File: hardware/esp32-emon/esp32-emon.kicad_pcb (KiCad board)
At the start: 2 copper layers, 86 x 35.2 mm, 11 parts, among them J1 SJ-3523-SMT-TR, J2 SJ-3523-SMT-TR, U1 ESP32-DEVKIT-V1

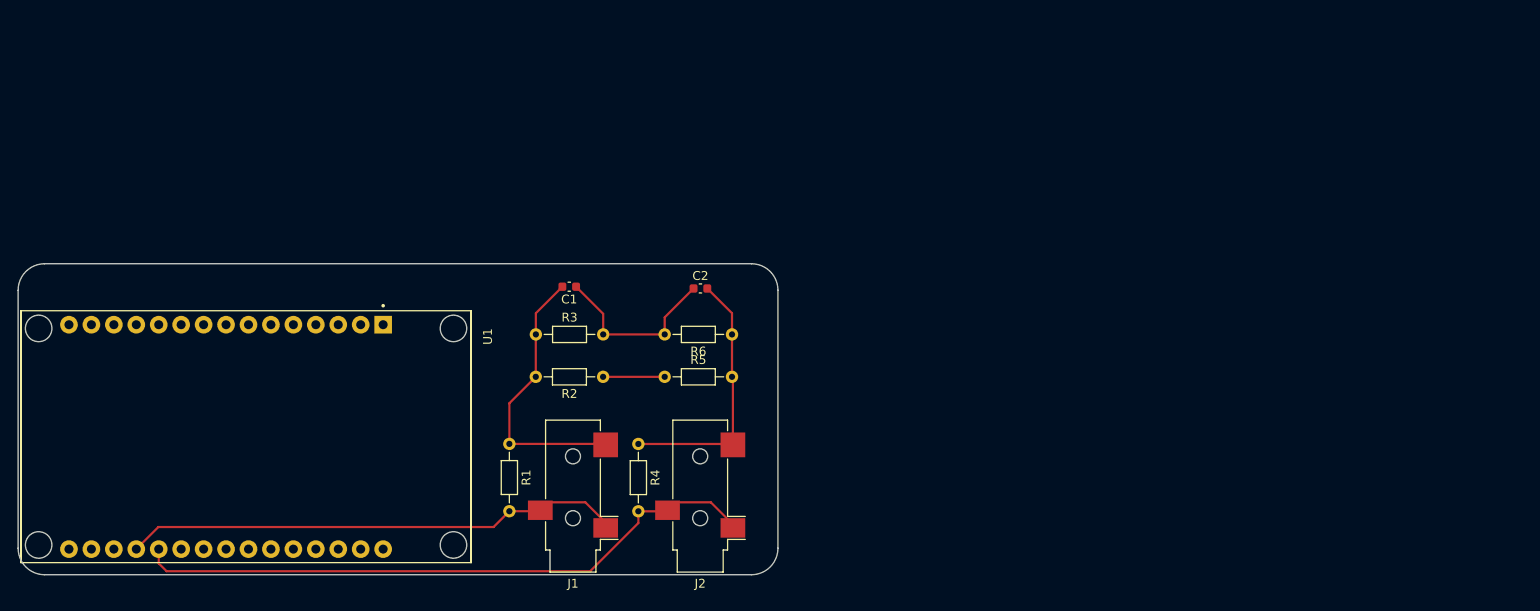
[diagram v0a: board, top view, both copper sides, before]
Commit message: Updates for v0.1
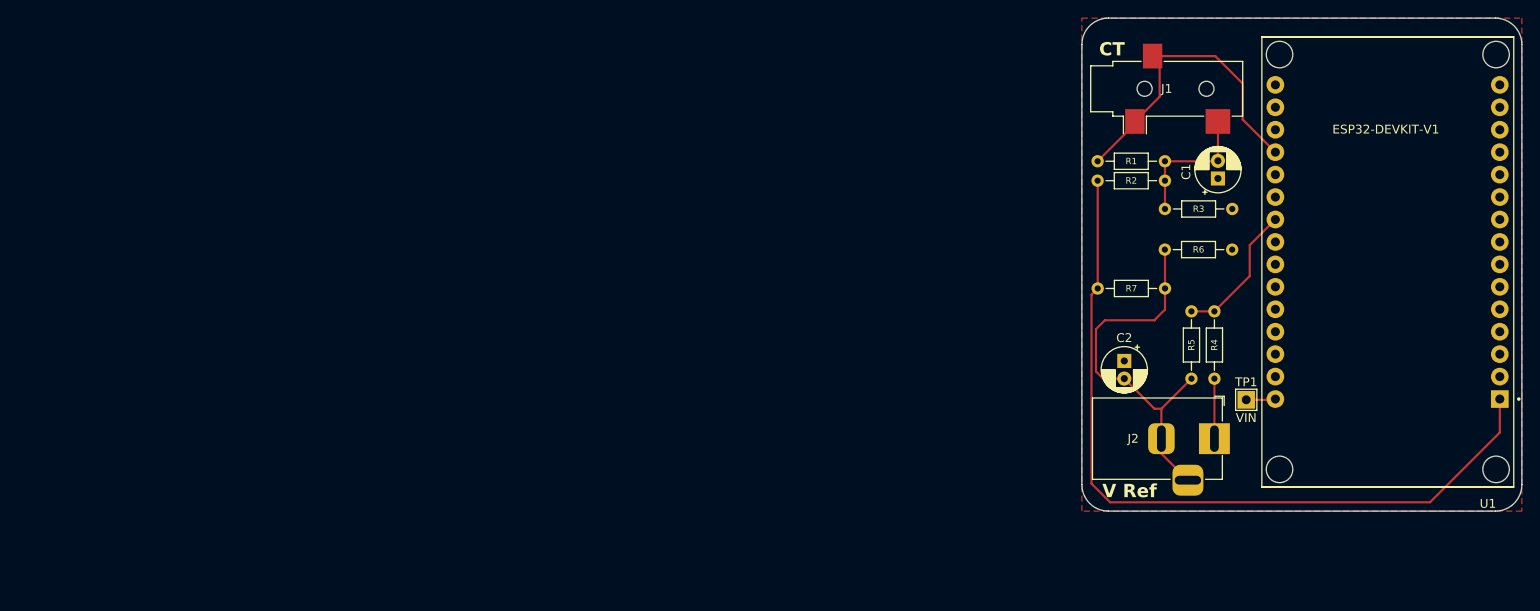
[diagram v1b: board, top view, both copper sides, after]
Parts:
- added R7: 470K, Resistor_THT:R_Axial_DIN0204_L3.6mm_D1.6mm_P7.62mm_Horizontal, F.Cu at (141.6, 56.6)
- added TP1: VIN, TestPoint:TestPoint_THTPad_2.0x2.0mm_Drill1.0mm, F.Cu at (158.4, 69.2)
- C1, C2: footprint Capacitor_SMD:C_0603_1608Metric -> Capacitor_THT:CP_Radial_D5.0mm_P2.00mm
- J2: value SJ-3523-SMT-TR -> Barrel_Jack; footprint Connector_Audio:Jack_3.5mm_CUI_SJ-3523-SMT_Horizontal -> Connector_BarrelJack:BarrelJack_Horizontal
- R4: value 18R -> 100K
- R5: value 470K -> 1K
- moved U1 130.7 mm to (174.4, 53.6), turned to 180 degrees
- moved J1 81.5 mm to (149.4, 34.0), turned to 90 degrees
- moved R1 80.8 mm to (149.2, 42.2), turned to 180 degrees
- moved C1 74.4 mm to (155.2, 44.2), turned to 90 degrees
- moved R3 72.6 mm to (149.2, 47.6)
- moved R4 66.9 mm to (154.8, 59.2)
- moved R2 60.2 mm to (141.6, 44.4), turned to 0 degrees
- moved R5 59.6 mm to (152.2, 66.8), turned to 90 degrees
- moved J2 58.6 mm to (154.8, 73.6), turned to 0 degrees
- moved R6 57.4 mm to (156.8, 52.2)
- moved C2 48.7 mm to (144.6, 64.8), turned to -90 degrees
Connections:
- R4 pad 1: Net-(C2-Pad2) -> /ADC1 CH5
- R4 pad 2: /ADC1 CH7 -> Net-(J2-Pad1)
- R5 pad 1: +3V3 -> Net-(C2-Pad2)
- R5 pad 2: Net-(C2-Pad2) -> /ADC1 CH5
- R6 pad 1: Net-(C2-Pad2) -> GND
- R6 pad 2: GND -> Net-(C2-Pad2)
- U1 pad 1: unconnected-(U1-3V3-Pad1) -> +3V3
- U1 pad 2: Net-(U1-GND-Pad2) -> GND
- U1 pad 20: /ADC1 CH7 -> unconnected-(U1-D35-Pad20)
- U1 pad 22: unconnected-(U1-D33-Pad22) -> /ADC1 CH5
- U1 pad 29: Net-(U1-GND-Pad2) -> GND
- U1 pad 30: unconnected-(U1-VIN-Pad30) -> Net-(U1-VIN)
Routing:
- net +3V3: track 6.97 -> 88.7 mm
- net /ADC1 CH7: track 72.4 -> 0.00 mm
- net /ADC1 CH6: track 56.9 -> 35.9 mm
- net GND: track 20.2 -> 0.00 mm
- net /ADC1 CH5: track 0.00 -> 15.9 mm
- net Net-(C1-Pad2): track 31.2 -> 16.4 mm
- net Net-(C2-Pad2): track 29.6 -> 43.6 mm
- net Net-(J2-Pad1): track 0.00 -> 6.79 mm
- net Net-(U1-VIN): track 0.00 -> 3.34 mm
- added copper zone on F.Cu, net GND
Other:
- board size 86 x 35.2 mm -> 49.8 x 55.8 mm
- board text added: "CT"
- board text added: "JALLERTON EMON V0.1"
- board text added: "V Ref"
